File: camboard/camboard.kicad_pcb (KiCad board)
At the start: 2 copper layers, 76.2 x 76.2 mm, 61 parts, among them J1 USB_microB_2040002-1, J2 Micro_SD_Card, J3 PPTC102LFBN-RC, J4 Conn_ARM_JTAG_SWD_20, J5 GS2, J6 Conn_01x25_Female, J7 Conn_01x25_Female, SW1 SW_DPDT_x2, SW2 SW_Push, SW3 SW_Push, SW4 SW_DPDT_x2, SW5 SW_DPDT_x2, U1 STM32F746VGT6, U2 MCP1703A-3302_SOT23, U3 FT230XS, Y1 SG-310SCN, Y2 NX3215SA

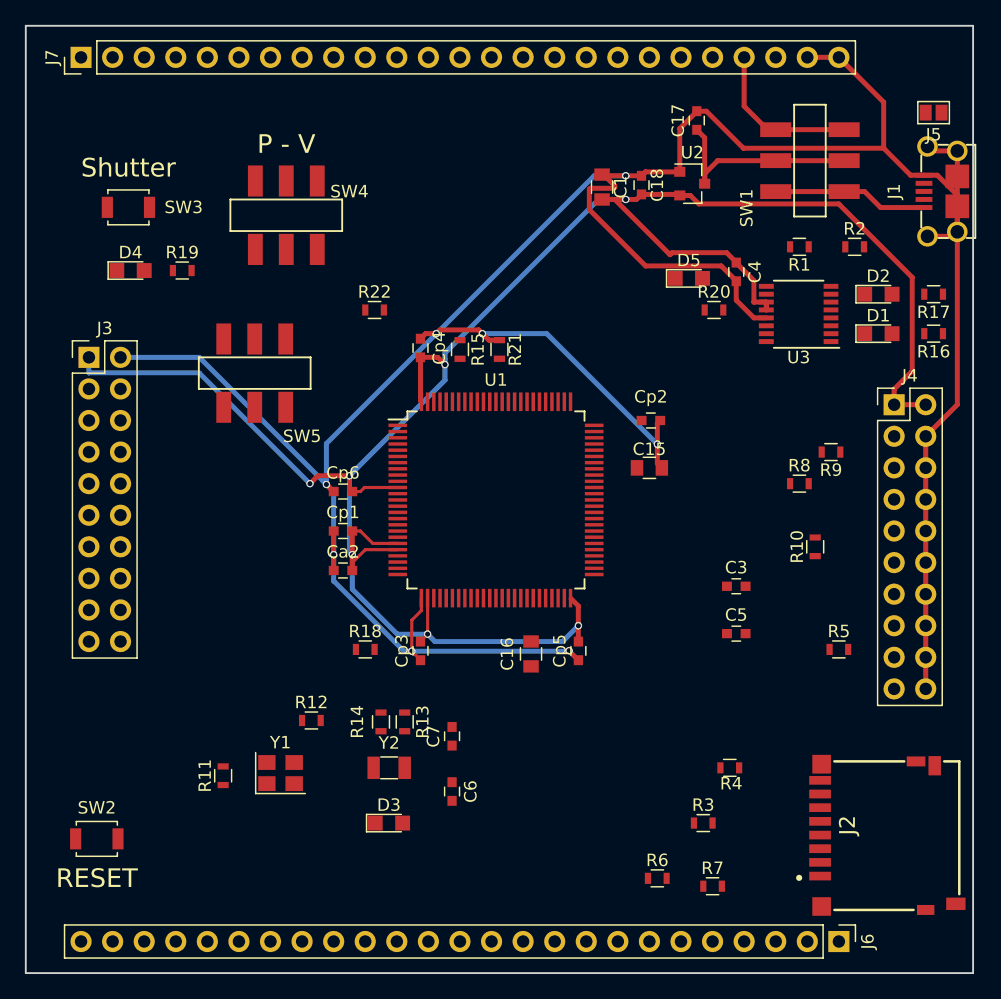
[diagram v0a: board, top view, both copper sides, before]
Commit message: The ladybug is happy
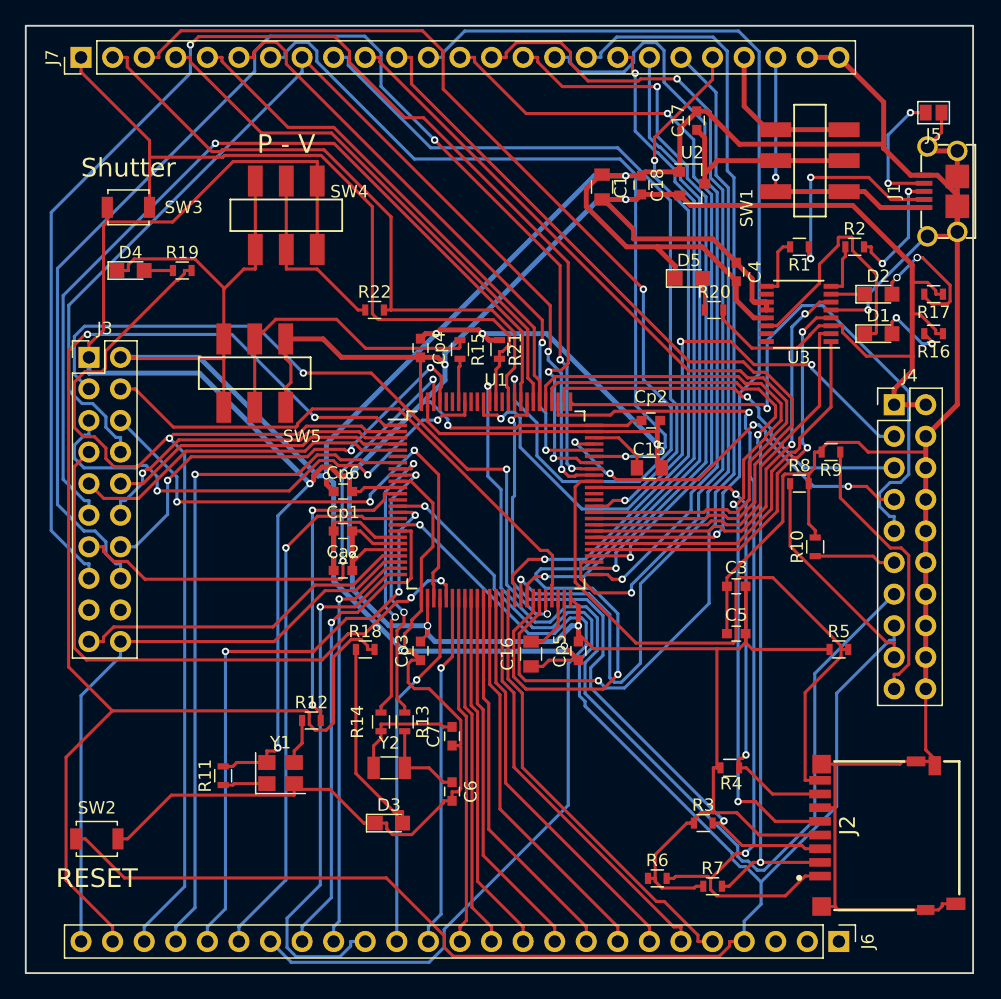
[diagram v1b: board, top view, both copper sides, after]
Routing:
- net GND: track 249.2 -> 473.1 mm, vias 8 -> 9
- net +3V3: track 179.2 -> 372.7 mm, vias 7 -> 9
- net /NRST: track 0.00 -> 138.4 mm, vias 0 -> 1
- net Net-(J6-Pad24): track 0.00 -> 111.0 mm, vias 0 -> 2
- net /DCMI_D1: track 0.00 -> 108.3 mm, vias 0 -> 3
- net /DCMI_D0: track 0.00 -> 104.6 mm, vias 0 -> 3
- net Net-(J6-Pad23): track 0.00 -> 89.4 mm, vias 0 -> 1
- net Net-(J7-Pad3): track 0.00 -> 87.0 mm, vias 0 -> 2
- net /CLK: track 0.00 -> 86.8 mm, vias 0 -> 2
- net Net-(J7-Pad17): track 0.00 -> 83.5 mm, vias 0 -> 1
- net Net-(J4-Pad13): track 0.00 -> 81.6 mm, vias 0 -> 1
- net Net-(J7-Pad18): track 0.00 -> 81.4 mm, vias 0 -> 2
- net Net-(J7-Pad12): track 0.00 -> 78.6 mm, vias 0 -> 1
- net /DCMI_D5: track 0.00 -> 72.7 mm, vias 0 -> 1
- net Net-(J7-Pad20): track 0.00 -> 71.4 mm, vias 0 -> 1
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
